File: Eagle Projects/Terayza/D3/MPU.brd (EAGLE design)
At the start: 80 x 80 mm, 41 parts, among them Q2 16MHz, Q3 16MHz, U2 MCP2551, U3 ATMEGA328P_TQFP, X1 5566-6, X2 5566-6

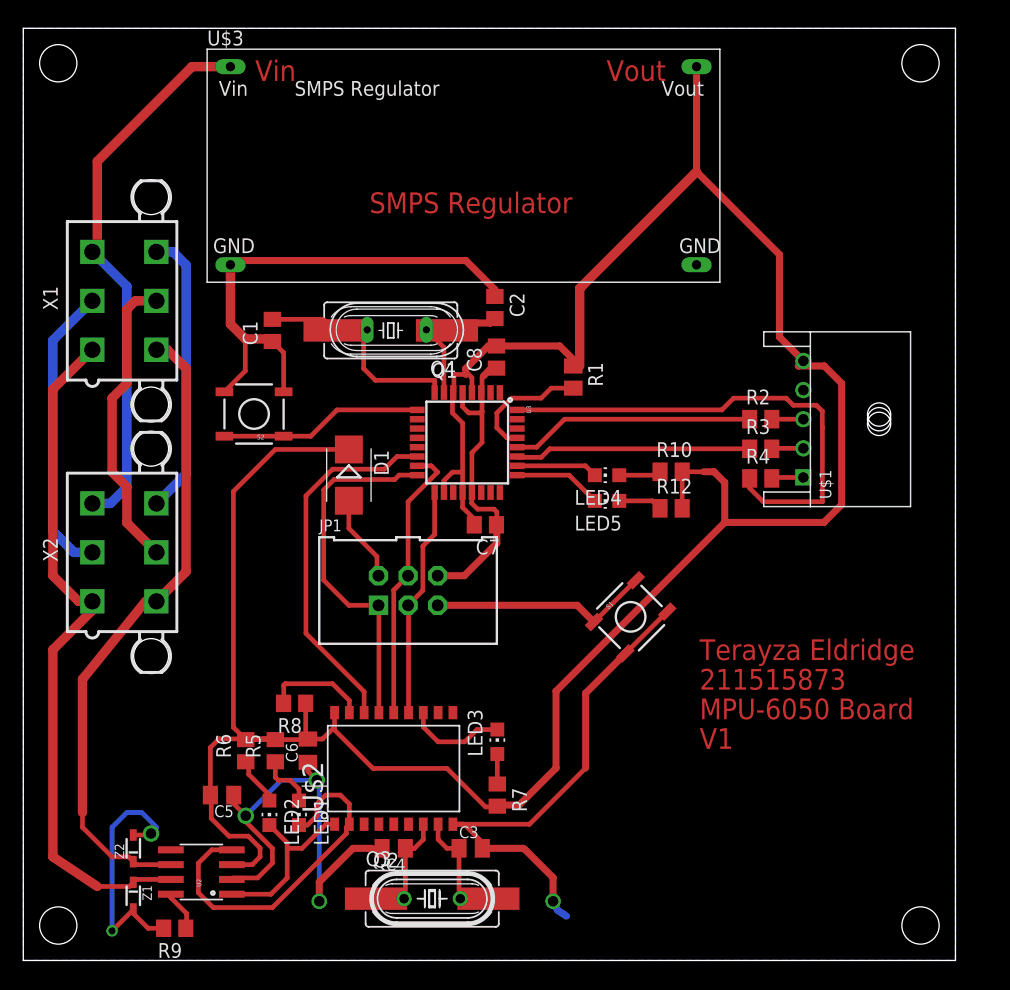
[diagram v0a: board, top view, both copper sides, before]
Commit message: Terayzas PCBS etched...
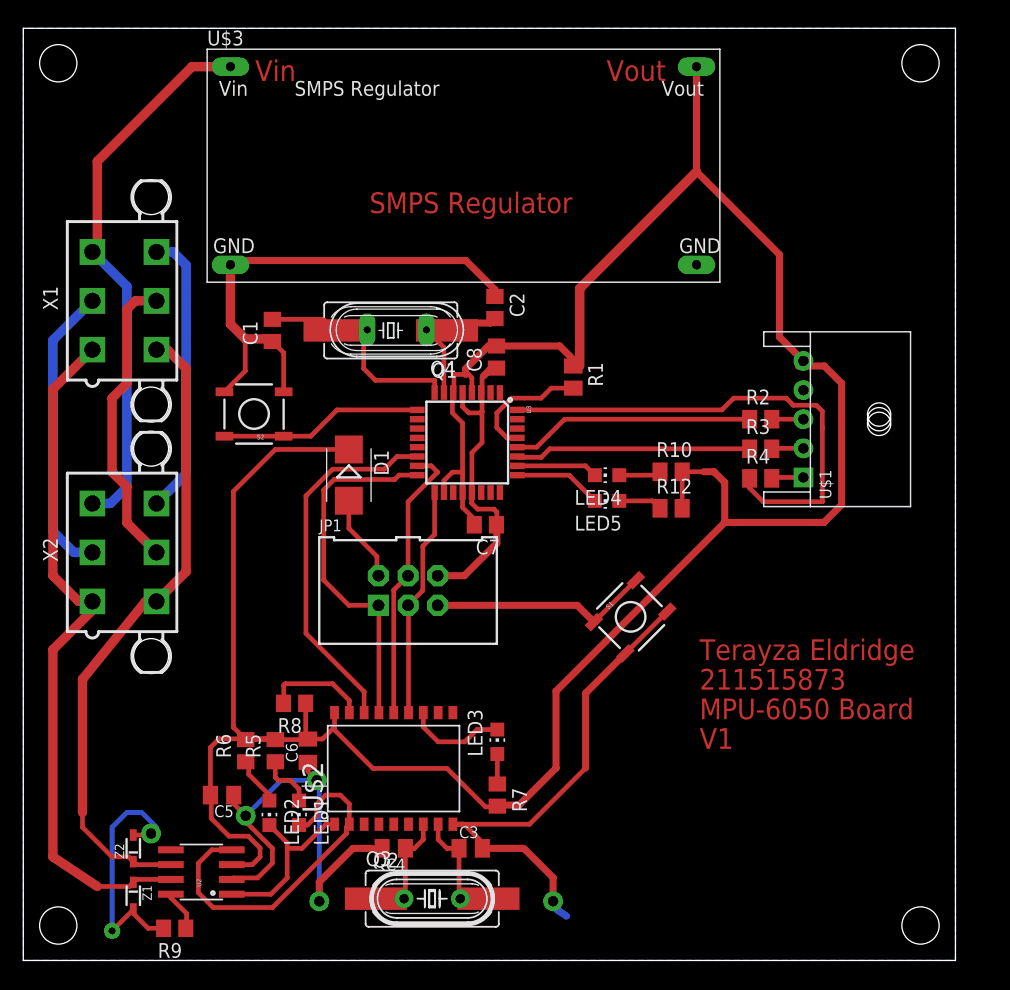
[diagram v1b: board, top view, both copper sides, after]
